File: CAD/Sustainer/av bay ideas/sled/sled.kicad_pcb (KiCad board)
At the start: 2 copper layers, 160.7 x 33 mm, 23 parts, among them J1 Conn_01x02, J2 Conn_01x02, SW1 SW_DIP_x01, SW2 SW_DIP_x01, SW3 SW_DIP_x01, SW4 SW_DIP_x01

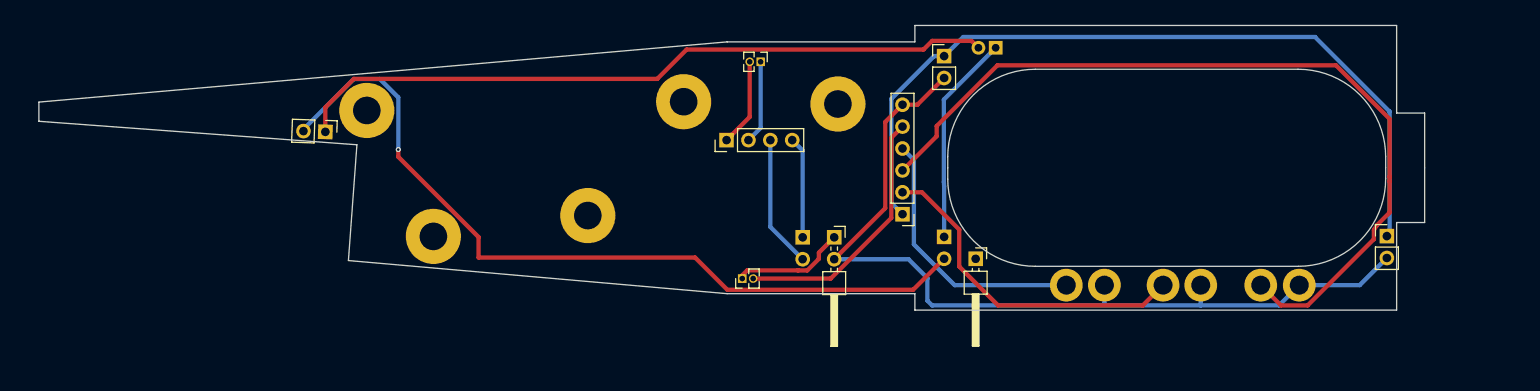
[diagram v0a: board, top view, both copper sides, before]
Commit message: new sled
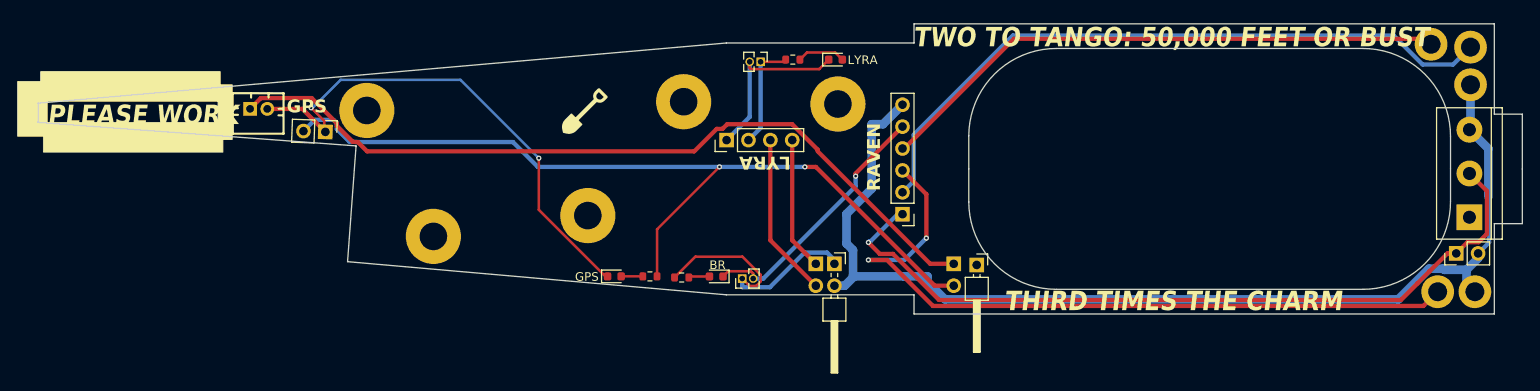
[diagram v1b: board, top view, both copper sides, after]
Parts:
- removed H7: MountingHole_Pad, MountingHole:MountingHole_2.2mm_M2_DIN965_Pad
- removed J1: Conn_01x02, Connector_PinHeader_2.54mm:PinHeader_1x02_P2.54mm_Vertical
- added D1: LED, LED_SMD:LED_0603_1608Metric, F.Cu at (168.1, 47.2)
- added D2: LED, LED_SMD:LED_0603_1608Metric, F.Cu at (154.3, 72.4)
- added D3: LED, LED_SMD:LED_0603_1608Metric, F.Cu at (142.5, 72.4)
- added R1: 1k, Resistor_SMD:R_0603_1608Metric, F.Cu at (163.2, 47.2)
- added R2: 1k, Resistor_SMD:R_0603_1608Metric, F.Cu at (150.3, 72.5)
- added R3: 1k, Resistor_SMD:R_0603_1608Metric, F.Cu at (146.6, 72.4)
- added SW5: SW_SPDT, TerminalBlock:TerminalBlock_bornier-3_P5.08mm, F.Cu at (241.7, 65.5)
- BT3: moved to F.Cu
- moved BT3 84.8 mm to (101.2, 53.0), turned to 0 degrees
- moved H6 50.7 mm to (237.2, 45.5)
- moved H10 45.1 mm to (241.8, 45.8), turned to -90 degrees
- moved H11 39.0 mm to (241.8, 50.2), turned to -90 degrees
- moved H8 20.5 mm to (238.0, 74.2), turned to 180 degrees
- moved H9 20.4 mm to (242.3, 74.2), turned to 180 degrees
- moved J2 8.29 mm to (240.2, 69.7), turned to 90 degrees
- moved SW2 3.43 mm to (165.9, 70.9)
- moved SW3 3.32 mm to (181.9, 70.9)
- moved SW1 3.07 mm to (168.0, 70.9)
- moved SW4 0.72 mm to (184.5, 71.1)
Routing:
- net Net-(BT3-+): track 24.4 -> 93.0 mm
- net /APO_BACKUP: track 39.1 -> 78.8 mm
- net /APOGEE: track 31.3 -> 66.8 mm
- net /BR_POS: track 102.2 -> 128.7 mm
- net Net-(BT3--): track 82.1 -> 60.0 mm, vias 0 -> 2
- net Net-(BT1-+): track 13.3 -> 29.5 mm
- net /MAIN: track 96.8 -> 85.7 mm, vias 0 -> 2
- net Net-(BT2--): track 10.2 -> 20.6 mm
- net Net-(GPS1-VIN): track 94.0 -> 100.0 mm, vias 1 -> 2
- net Net-(D1-A): track 0.00 -> 5.60 mm
- net Net-(LYRA1-SW+): track 15.4 -> 19.1 mm
- net Net-(LYRA1-SW-): track 11.8 -> 15.5 mm
- net Net-(BT2-+): track 9.67 -> 12.7 mm
- net Net-(D3-A): track 0.00 -> 2.51 mm
- net Net-(D2-A): track 0.00 -> 2.45 mm
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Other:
- board size 160.7 x 33 mm -> 172.2 x 33.7 mm
- board text added: "BR"
- board text added: "GPS"
- board text added: "LYRA"
- board text added: "MACH 3 50,000 FEET AND BACK"
- board text added: "PLEASE WORK"
- board text added: "POLARIS SPACE"
- board text added: "RAVEN"
- board text added: "THIRD TIMES THE CHARM"
- board text added: "TWO TO TANGO: 50,000 FEET OR BUST"
- board text added: "TWO TO TANGO: MACH 3 OR BUST"
